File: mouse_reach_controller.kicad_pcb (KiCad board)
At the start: 2 copper layers, 158.8 x 57.2 mm, 115 parts, among them J1 AUDIO_JACK_3.5MM, P1 HEADER_02X05_LATCH, P2 HEADER_02X05_LATCH, P3 HEADER_02X05_LATCH, P4 PWR_JACK_2.1x5.5_SMD_RA, P5 BNC_DOUBLE_RA, P6 BNC_DOUBLE_RA, P7 BNC_DOUBLE_RA, T1 TERM_BLK_HDR_2POS_90DEG_0.2IN, T2 TERM_BLK_HDR_4POS_90DEG_0.2IN, U1 TMC429, U10 SGTL5000, U11 RT9076-15GV, U12 74LVC1G125GS, U13 74LVC1G125GS, U14 TMC424, U15 74LVC1G125GS, U16 74LVC1G125GS, U17 74LVC1G125GS, U18 74LVC1G125GS, U19 74LVC1G125GS, U2 SN65LVDM050QDRQ1, U20 74LVC1G125GS, U3 74LVC1G125GS, U4 SN65LVDM050QDRQ1, U5 74LVC1G125GS, U6 SN65LVDM050QDRQ1, U7 74LVC1G125GS, U8 ZXMS6006SG, U9 RT9076-15GV

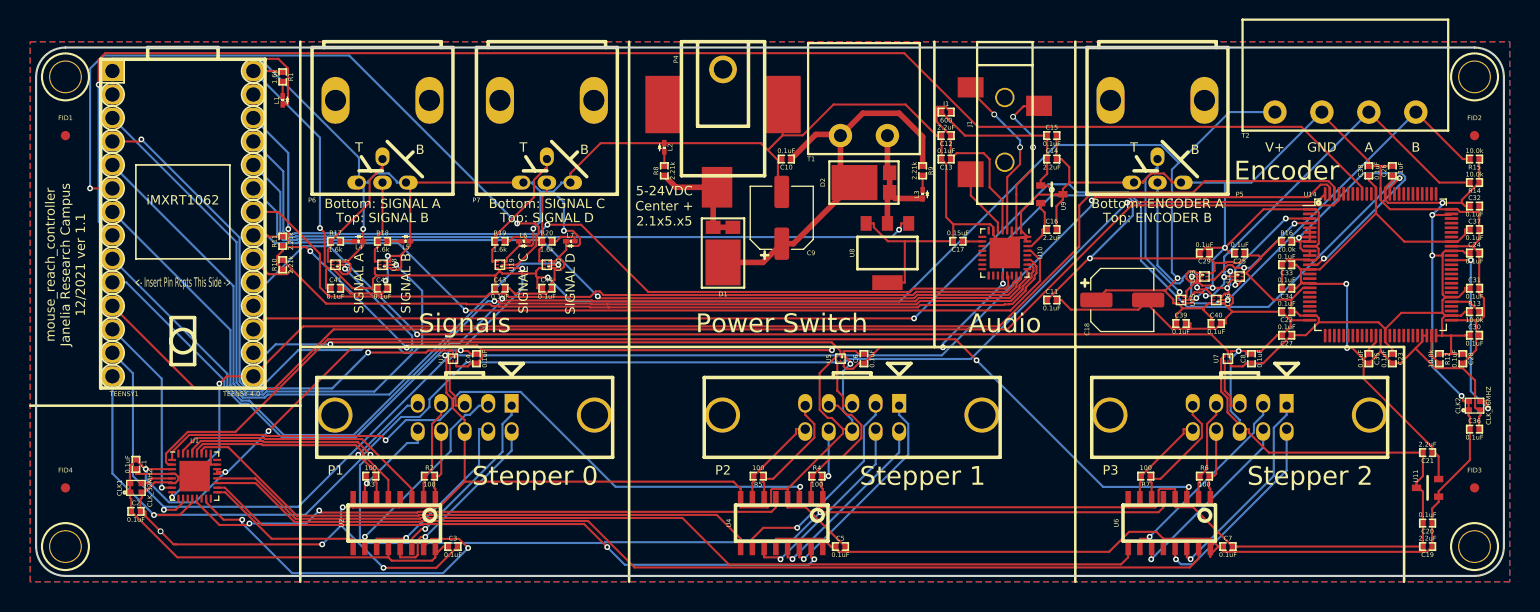
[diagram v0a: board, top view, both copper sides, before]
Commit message: Export schematic and board files for manufacturing and assembly
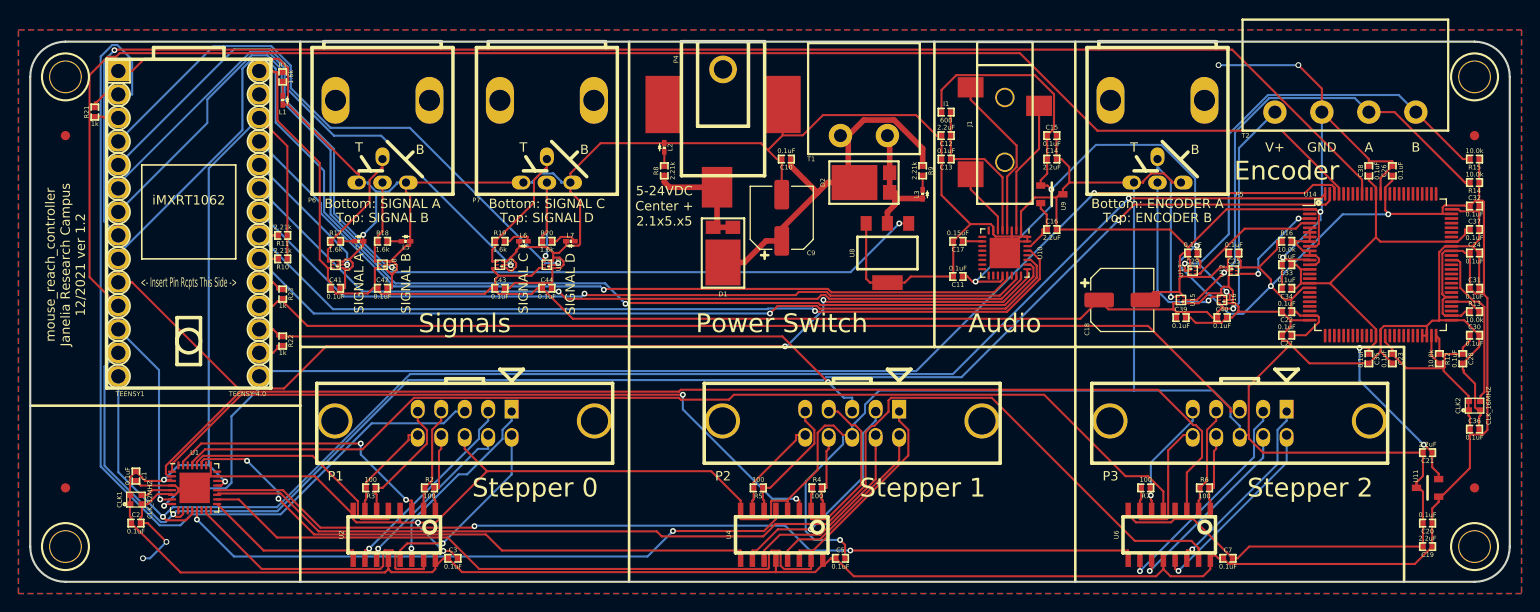
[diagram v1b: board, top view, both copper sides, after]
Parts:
- removed C4, C6, C8: 0.1uF, mouse_reach_controller:SM0402
- removed U3, U5, U7: 74LVC1G125GS, mouse_reach_controller:SOT1202
- added R21: 1k, mouse_reach_controller:SM0402, F.Cu at (75.6, 58.4)
- added R22: 1k, mouse_reach_controller:SM0402, F.Cu at (95.9, 83.2)
- added R23: 1k, mouse_reach_controller:SM0402, F.Cu at (95.9, 78.1)
- C18, C9: footprint mouse_reach_controller:CP_Elec_6.3x7.7_WURTH -> mouse_reach_controller:CP_Elec_6.3x8.3_PAN
- TEENSY1: value VAL** -> TEENSY_4.0_PIN_RECEPTACLES
- moved C11 10.5 mm to (168.9, 76.2), turned to 270 degrees
- moved U13 1.42 mm to (194.3, 75.6)
- moved C1 1.27 mm to (80.0, 97.8)
- moved C2 1.27 mm to (80.0, 102.9)
- moved C29 1.27 mm to (194.3, 73.7)
- moved C3 1.27 mm to (114.3, 106.7)
- moved C5 1.27 mm to (156.2, 106.7)
- moved C7 1.27 mm to (198.1, 106.7)
- moved CLK1 1.27 mm to (80.0, 100.3)
- moved R2 1.27 mm to (111.8, 99.1)
- moved R3 1.27 mm to (105.4, 99.1)
- moved R4 1.27 mm to (153.7, 99.1)
- moved R5 1.27 mm to (147.3, 99.1)
- moved R6 1.27 mm to (195.6, 99.1)
- moved R7 1.27 mm to (189.2, 99.1)
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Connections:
- P1 pad 5: /stepper_controller/stepper_driver_interface_0/UART_BUFFERED -> /UART_CPU_RX_0
- P2 pad 5: /stepper_controller/stepper_driver_interface_1/UART_BUFFERED -> /UART_CPU_RX_1
- P3 pad 5: /stepper_controller/stepper_driver_interface_2/UART_BUFFERED -> /UART_CPU_RX_2
- TEENSY1 pad 0: (no net) -> /UART_CPU_RX_0
- TEENSY1 pad 1: /UART_0 -> /UART_CPU_TX_0
- TEENSY1 pad 14: /UART_1 -> /UART_CPU_TX_1
- TEENSY1 pad 15: /ENCODER_INVERT -> /UART_CPU_RX_1
- TEENSY1 pad 16: (no net) -> /UART_CPU_RX_2
- TEENSY1 pad 17: /UART_2 -> /UART_CPU_TX_2
- TEENSY1 pad 2: /SIGNAL_A -> /SIGNAL_D
- TEENSY1 pad 22: /POWER_SWITCH_ENABLE -> /SIGNAL_A
- TEENSY1 pad 3: /SIGNAL_B -> /SIGNAL_C
- TEENSY1 pad 4: /SIGNAL_C -> /SIGNAL_B
- TEENSY1 pad 5: /SIGNAL_D -> /POWER_SWITCH_ENABLE
- U14 pad 86: /ENCODER_INVERT -> (no net)
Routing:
- net /ENCODER_INVERT: track 147.4 -> 0.00 mm, vias 2 -> 0
- net /UART_2: track 112.2 -> 0.00 mm, vias 1 -> 0
- net /UART_CPU_RX_2: track 0.00 -> 111.7 mm
- net /UART_CPU_RX_0: track 0.00 -> 104.7 mm
- net /UART_CPU_RX_1: track 0.00 -> 68.9 mm, vias 0 -> 1
- net /UART_1: track 64.8 -> 0.00 mm, vias 1 -> 0
- net /UART_0: track 60.3 -> 0.00 mm, vias 1 -> 0
- net /SIGNAL_A: track 67.8 -> 15.8 mm, vias 2 -> 1
- net /GND: track 798.4 -> 750.7 mm, vias 19 -> 10
- net /POWER_SWITCH_ENABLE: track 77.7 -> 112.0 mm
- net /VDD: track 505.7 -> 471.6 mm, vias 15 -> 7
- net /encoder_interface/VDD_PULLUP: track 36.0 -> 8.68 mm, vias 2 -> 0
- net /~ENCODER_CS: track 145.5 -> 169.1 mm
- net /SIGNAL_C: track 78.7 -> 59.5 mm, vias 2 -> 1
- net /VCC: track 186.9 -> 168.9 mm, vias 3 -> 1
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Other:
- board size 158.8 x 57.2 mm -> 160 x 58.4 mm
- board text added: "mouse_reach_controller Janelia Research Campus 12/2021 ver 1.2"
- board text removed: "mouse_reach_controller Janelia Research Campus 12/2021 ver 1.1"
